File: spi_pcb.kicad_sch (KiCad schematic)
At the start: 22 parts, among them J1 GPIO, J2 PWR, U1 imported:LMZ23605TZ

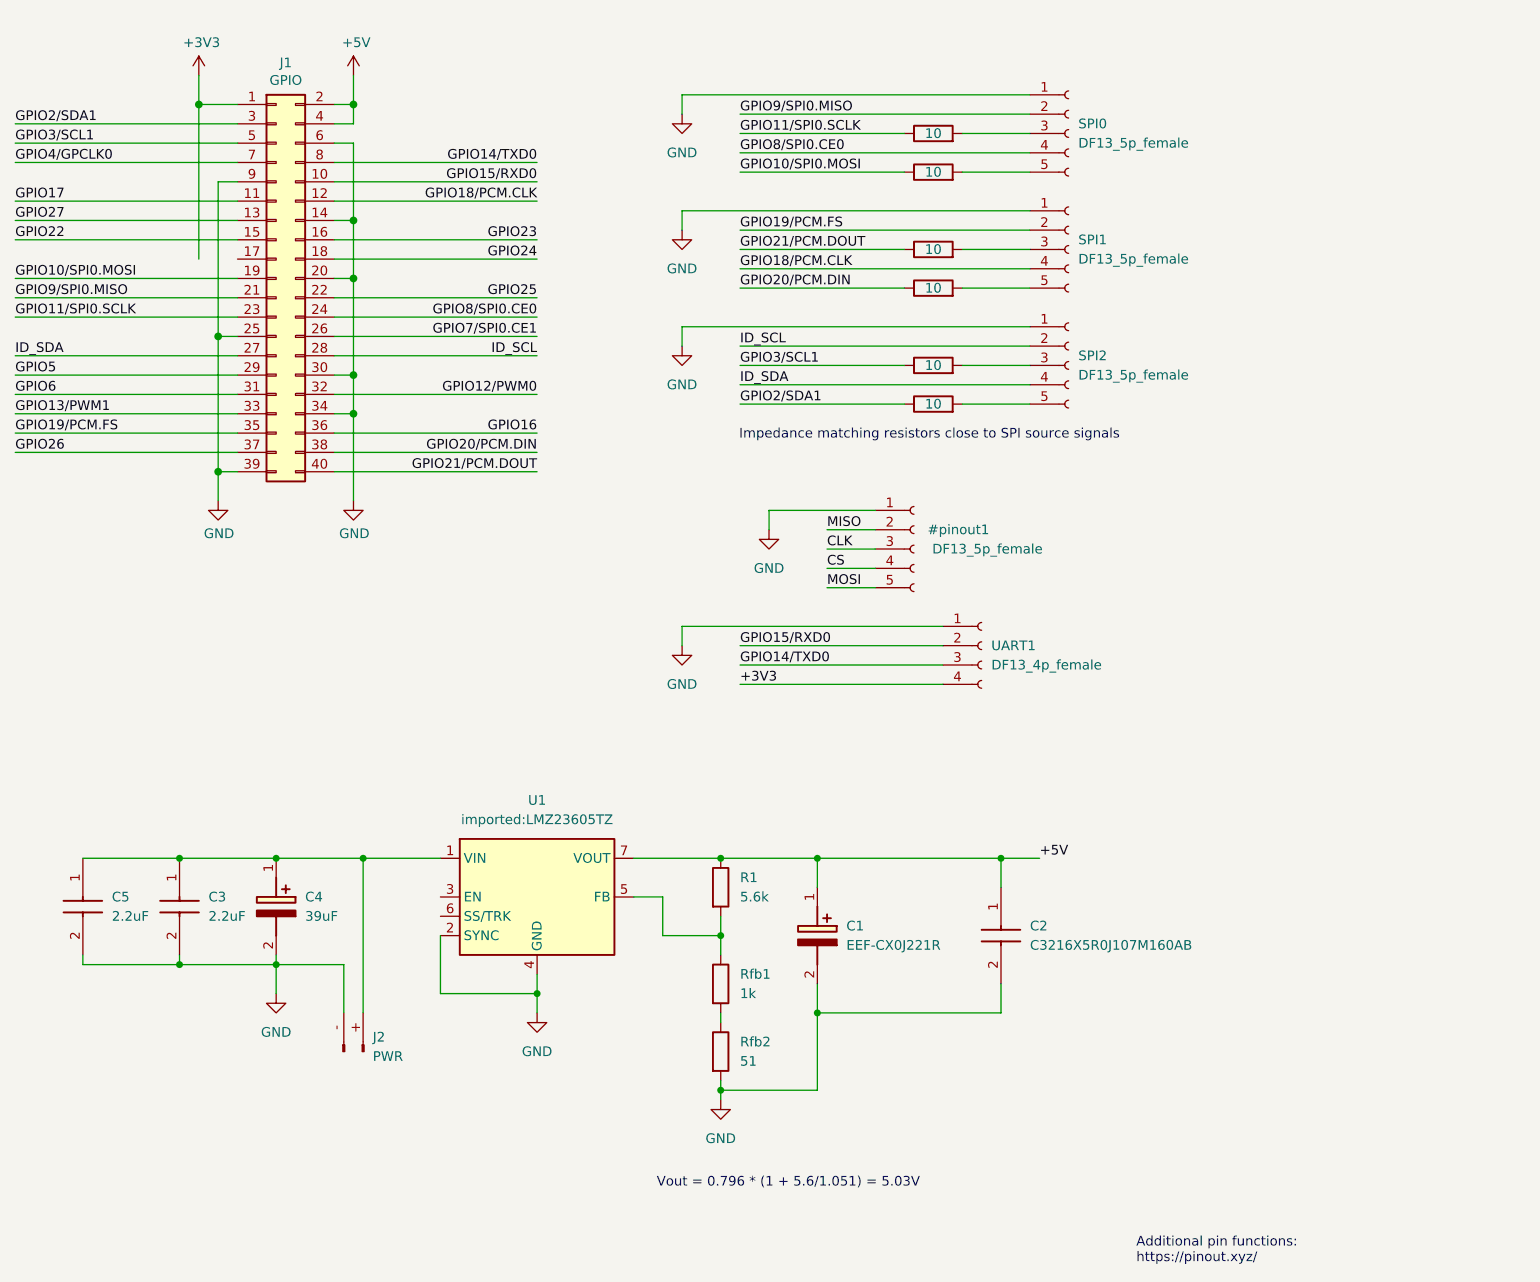
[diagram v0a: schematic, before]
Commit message: Add information to schematic
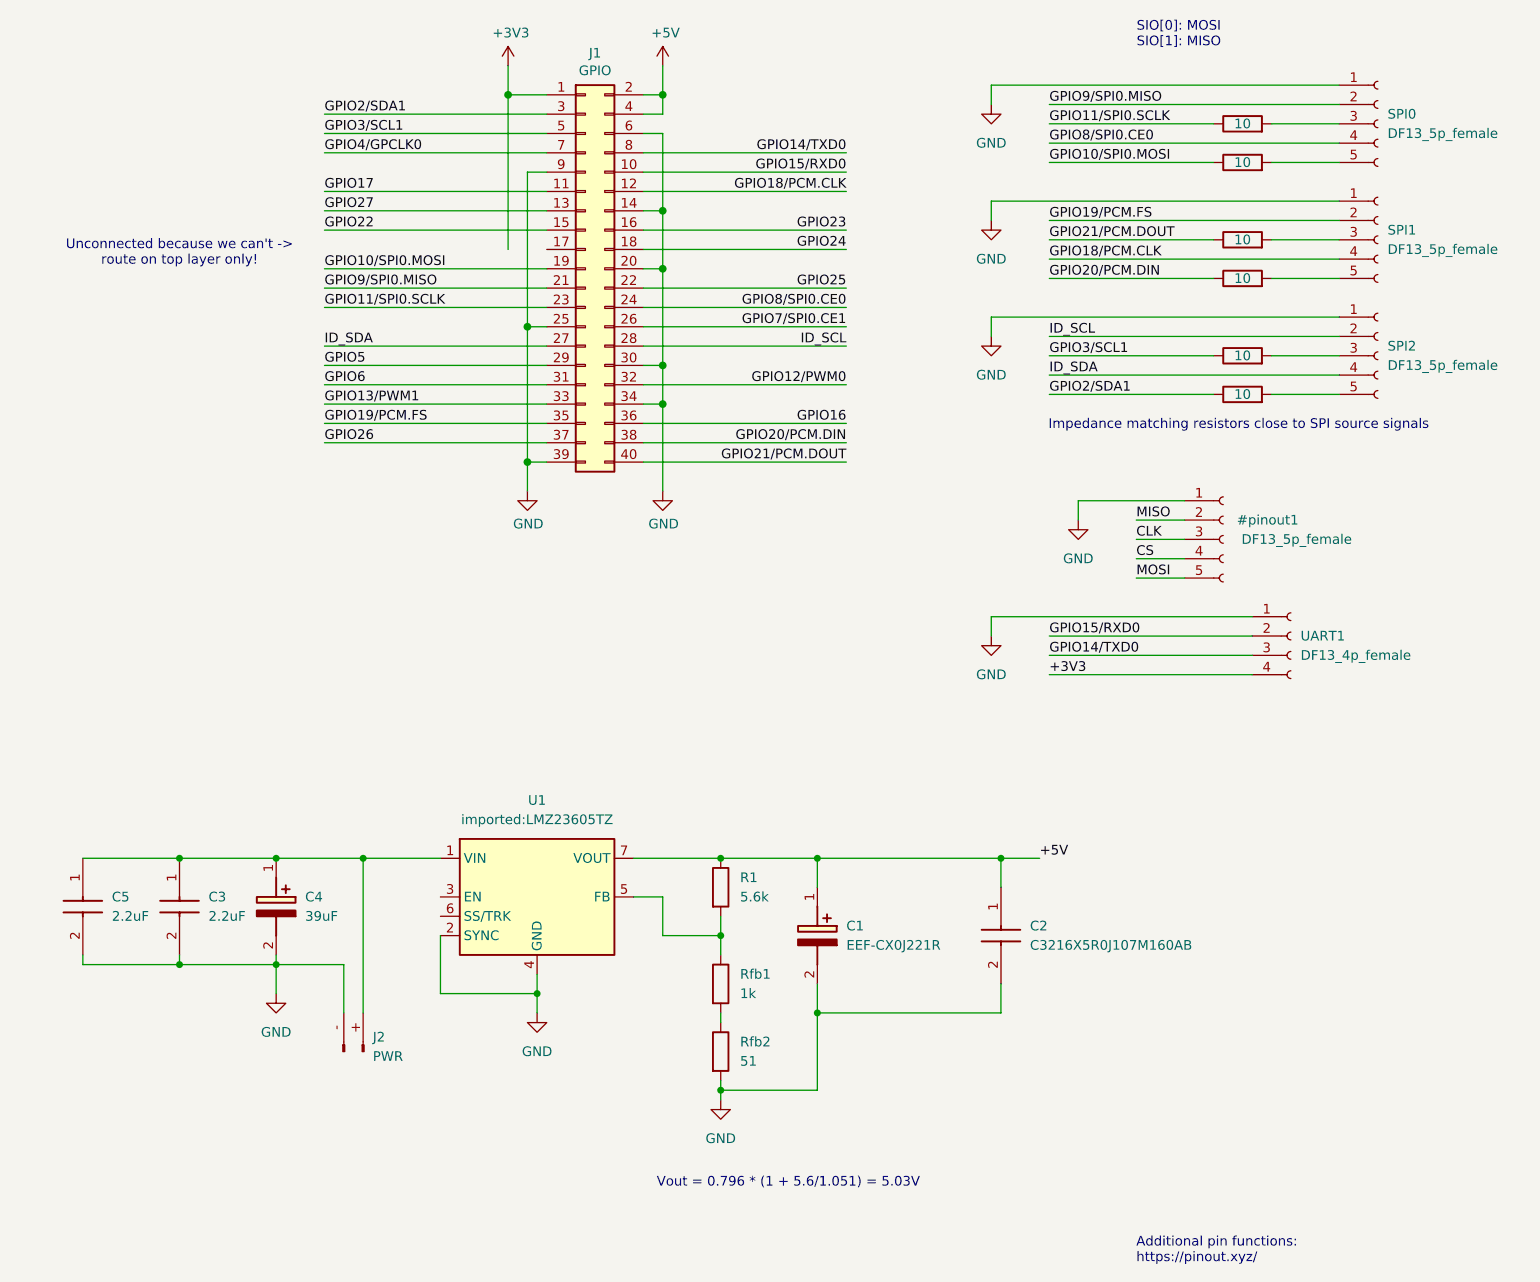
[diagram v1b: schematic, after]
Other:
- note added: "SIO[0]: MOSI SIO[1]: MISO"
- note added: "Unconnected because we can't -> route on top layer only!"
- moved on the sheet: J1, SPI0, SPI1, SPI2, UART1
